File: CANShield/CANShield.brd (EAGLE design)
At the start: 96.5 x 128.3 mm, 69 parts, among them IC1 7805DT, IC2 74LVC2G125DCT, IC3 ILD213T, IC4 ILD213T, IC5 ILD213T, J2 POWERPOLE_POWER25A_HORIZONTAL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, Q1 MOSFET-NCHANNELFDD8780, Q2 MOSFET-NCHANNELFDD8780, Q3 MOSFET-NCHANNELFDD8780, Q4 MOSFET-NCHANNELFDD8780, Q5 MOSFET-NCHANNELFDD8780, Q6 MOSFET-NCHANNELFDD8780, Q7 MOSFET-NCHANNELBSS123LT1G, Q8 BSS123, U5 MCP2551, X1 DB9 Plug

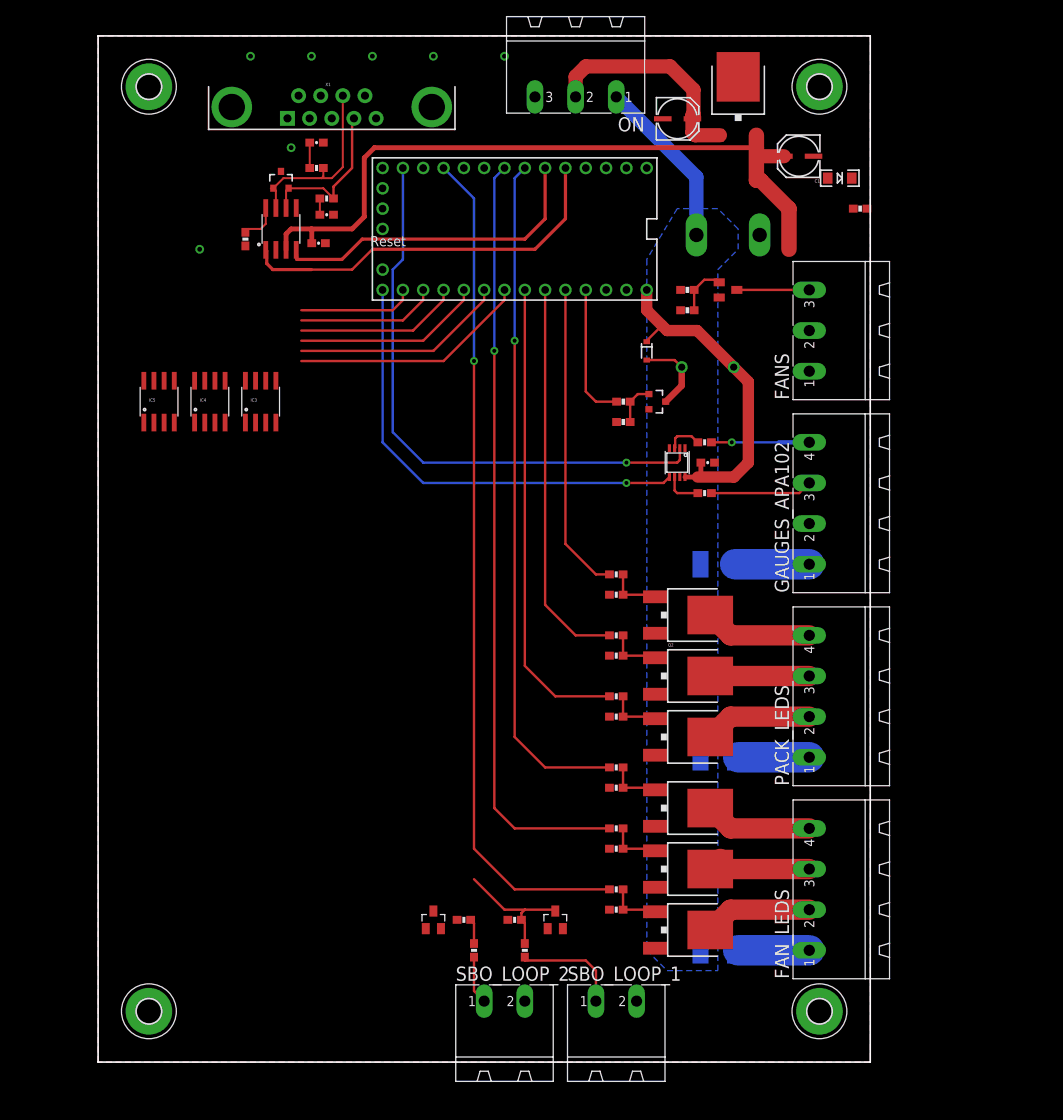
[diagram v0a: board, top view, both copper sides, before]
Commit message: precharge progress
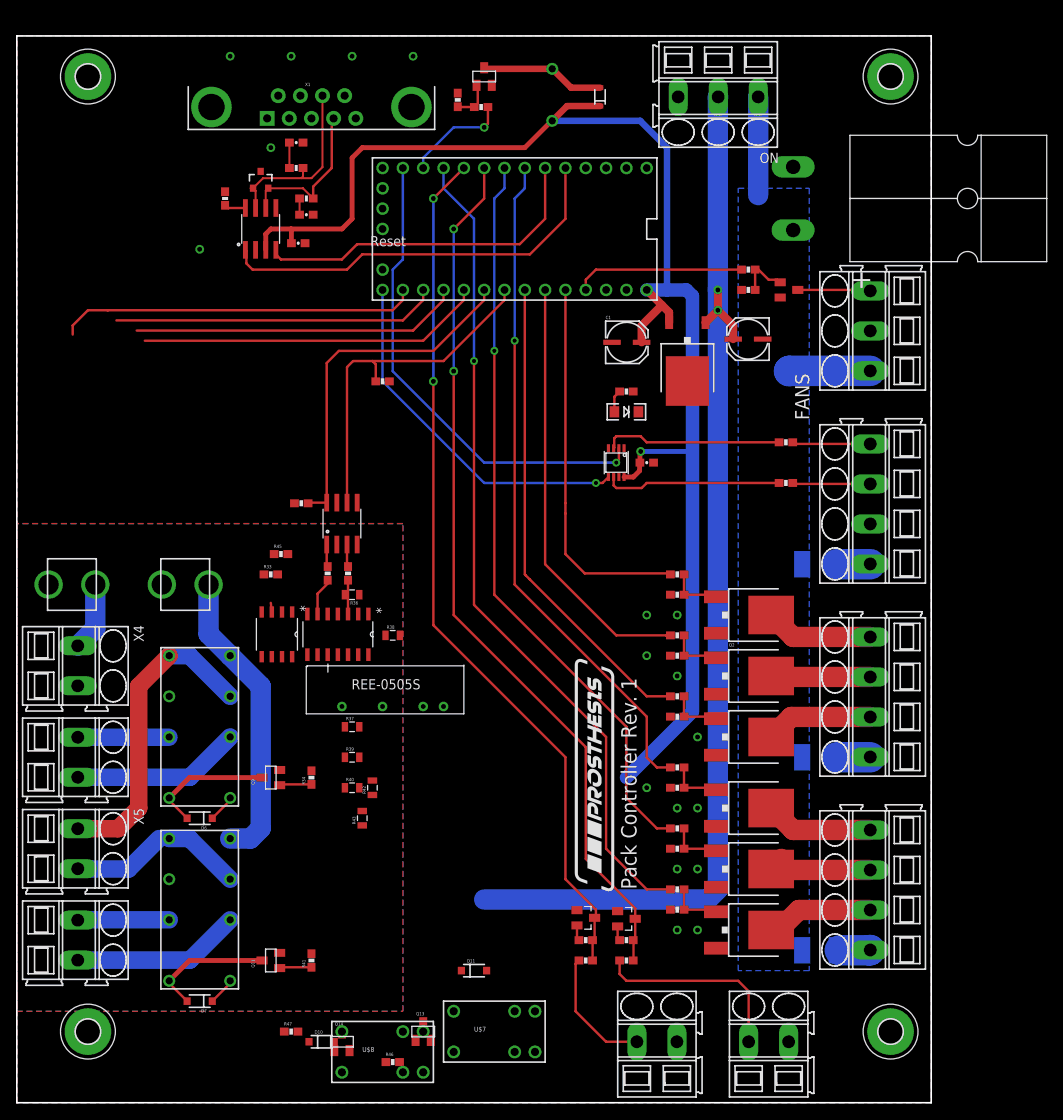
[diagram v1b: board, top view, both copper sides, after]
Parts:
- removed IC4, IC5: ILD213T, SparkFun-DiscreteSemi:SO08
- added 74HC125M: MM74HC125M, Fairchild_By_element14_Batch_1:SOIC127P600X175-14N
- added D10, D11, D6, D7: (no value), SparkFun-DiscreteSemi:SOD-123
- added LM393M: LM393M, Fairchild_By_element14_Batch_1:SOIC127P600X180-8N
- added PRECHARGE_FUSE: FUSEX20MM, SparkFun-Passives:FUSE_5MM
- added PRECHARGE_RELAY, PRECHARGE_RELAY1: DS2Y-S-DC5V, relay:DS2Y
- added Q11, Q13, Q14, Q9: IRLML6344TRPBF, SparkFun-DiscreteSemi:SOT23
- added R23, R24, R25, R26: 10K, SparkFun-Passives:0603-RES
- added R33, R45: 100k, SparkFun-Resistors:0603-RES
- added R34, R41, R46, R47: 10k, SparkFun-Resistors:0603-RES
- added R36, R37, R42: 470k, SparkFun-Resistors:0805
- added R38, R43: 13K, SparkFun-Resistors:0805
- added R39: 110k, SparkFun-Resistors:0805
- added R40: 12K, SparkFun-Resistors:0805
- added U$4: (no value), prosthesis:PROS_LOGO
- added U$5: REE-0505S, grant:REE-0505S
- added U$7, U$8: RELAY-2G5Q, SparkFun-Electromechanical:RELAY-G5V
- added X2, X3, X4, X5: SMKDSP_1,5/2, con-phoenix-smkdsp:SMKDSP_1,5/2
- FANS, ON: value MSTBA3 -> SMKDSP_1,5/3; device con-phoenix-508:MSTBA3 -> con-phoenix-smkdsp:SMKDSP_1,5/3
- FAN_LEDS, GAUGES_APA102, PACK_LEDS: value MSTBA4 -> SMKDSP_1,5/4; device con-phoenix-508:MSTBA4 -> con-phoenix-smkdsp:SMKDSP_1,5/4
- Q7: device SparkFun-DiscreteSemi:SOT23-3 -> SparkFun-DiscreteSemi:SOT23
- R10, R12, R13: device SparkFun-Resistors:0603-RES -> SparkFun-Resistors:0603-RES@1
- SBO_LOOP_1, SBO_LOOP_2: value MSTBA2 -> SMKDSP_1,5/2; device con-phoenix-508:MSTBA2 -> con-phoenix-smkdsp:SMKDSP_1,5/2
- moved Q7 46.0 mm to (44.5, 111.8), turned to 0 degrees
- moved R30 45.3 mm to (41.1, 108.8), turned to 270 degrees
- moved R29 40.9 mm to (44.1, 108.0), turned to 180 degrees
- moved D1 39.6 mm to (62.2, 69.8)
- moved SG1 39.2 mm to (53.0, 109.5), turned to 270 degrees
- moved R22 37.1 mm to (62.2, 72.4), turned to 0 degrees
- moved IC1 33.6 mm to (69.8, 76.2), turned to 180 degrees
- moved D2 32.3 mm to (58.9, 109.2), turned to 90 degrees
- moved C1 31.4 mm to (62.2, 78.7), turned to 0 degrees
- moved C4 29.3 mm to (77.5, 78.7), turned to 180 degrees
- moved ON 20.9 mm to (76.2, 109.2)
- moved D4 19.1 mm to (57.1, 6.60), turned to 270 degrees
- moved SBO_LOOP_1 19.1 mm to (80.0, -8.89)
- moved SBO_LOOP_2 19.1 mm to (66.0, -8.89)
- moved IC3 18.3 mm to (26.7, 55.9)
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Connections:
- removed net CHARGED_1: U$1.18/A4
- removed net CHARGING_1: U$1.19/A5
- new net 96V_IN_FUSED: PRECHARGE_FUSE.1, PRECHARGE_RELAY.8, PRECHARGE_RELAY1.8, R37.2
- new net CAP_CHARGE_REF: LM393M.2, R39.1, R40.2
- new net CAP_CHARGE_V_CURR_1: LM393M.3, R36.1, R38.2
- new net CAP_CHARGE_V_CURR_2: R42.1, R43.2
- new net CHARGE_1: IC3.6, R23.1, U$1.19/A5
- new net CHARGE_2: IC3.8, R26.1, U$1.18/A4
- new net CHARGE_ISO_1: 74HC125M.3, R25.2
- new net CHARGE_ISO_2: 74HC125M.6, R24.2
- new net CONTACT_EN_1: Q13.1, R46.1
- new net CONTACT_EN_2: Q14.1, R47.1
- new net GNDI: IC3.2, IC3.4, U$5.-VOUT, X4.2
- new net N$30: R37.1, R39.2
- new net N$31: 74HC125M.12, 74HC125M.9, LM393M.7, R45.2
- new net N$32: IC3.3, R25.1
- new net N$33: D10.A, Q14.3, U$8.9
- new net N$34: IC3.1, R24.1
- new net N$35: D11.A, Q13.3, U$7.9
- new net N$36: 74HC125M.8
- new net N$37: 74HC125M.11
- new net N$38: U$7.5, U$7.6
- new net N$39: U$8.5, U$8.6
- new net N$40: PRECHARGE_RELAY.13, X2.1
- new net N$41: PRECHARGE_RELAY1.13, X3.1
- new net N$42: PRECHARGE_FUSE.3, X4.1
- new net PRECHARGE_EN_1: Q9.1, R34.1
- new net PRECHARGE_EN_2: Q11.1, R41.1
- new net PRECHARGE_OUT_1: PRECHARGE_RELAY.6, PRECHARGE_RELAY.9, R36.2, X5.1
- new net PRECHARGE_OUT_2: PRECHARGE_RELAY1.6, PRECHARGE_RELAY1.9, R42.2, X5.2
- new net PRECHARGE_RESISTOR_IN: PRECHARGE_RELAY.4, X2.2
- new net PRECHARGE_RESISTOR_IN1: PRECHARGE_RELAY1.4, X3.2
- new net PRECH_DRAIN: D6.A, PRECHARGE_RELAY.16, Q9.3
- new net PRECH_DRAIN1: D7.A, PRECHARGE_RELAY1.16, Q11.3
- new net PRECH_STATE_TO_BUFF: 74HC125M.2, 74HC125M.5, LM393M.1, R33.2
- net +12V: now also D10.C, D11.C, U$7.2, U$8.2
- net +5V: now also R23.2, R26.2, U$5.+VIN
- net 5V: now also 74HC125M.14, D6.C, D7.C, LM393M.8, PRECHARGE_RELAY.1, PRECHARGE_RELAY1.1, R33.1, R45.1, U$5.+VOUT
- net BUZZER: now also U$1.10; no longer U$1.23/A9
- net FAN_PWM: now also U$1.23/A9; no longer U$1.10
- net GND: now also 74HC125M.1, 74HC125M.10, 74HC125M.13, 74HC125M.4, 74HC125M.7, IC3.5, IC3.7, LM393M.4, PRECHARGE_RELAY.11, PRECHARGE_RELAY1.11, Q11.2, Q13.2, Q14.2, Q9.2, R34.2, R38.1, R40.1, R41.2, R43.1, R46.2, R47.2, U$5.-VIN, U$7.10, U$8.10
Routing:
- net VCC: track 28.6 -> 137.9 mm, vias 0 -> 2
- net SBO_SENSE_2: track 3.13 -> 109.4 mm, vias 0 -> 2
- net SBO_SENSE_1: track 16.4 -> 110.2 mm, vias 0 -> 2
- net +5V: track 137.1 -> 182.0 mm, vias 0 -> 1
- net CHARGE_1: track 0.00 -> 44.1 mm
- net CHARGE_2: track 0.00 -> 44.0 mm
- net PRECHARGE_OUT_1: track 0.00 -> 39.0 mm
- net 96V_IN_FUSED: track 0.00 -> 37.5 mm
- net ACTIVE_2: track 14.5 -> 45.0 mm
- net CHARGING_1: track 29.8 -> 0.00 mm
- net CHARGED_1: track 26.8 -> 0.00 mm
- net CHARGED_2: track 17.6 -> 40.7 mm
- net PRECHARGE_OUT_2: track 0.00 -> 22.7 mm
- net PRECHARGE_RESISTOR_IN1: track 0.00 -> 21.1 mm
- net PRECHARGE_RESISTOR_IN: track 0.00 -> 21.1 mm
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- added copper zone on layer 1, net GNDI
- added copper zone on layer 16, net GNDI
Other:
- board size 96.5 x 128.3 mm -> 114.3 x 133.3 mm
- board text added: "Pack Controller Rev. 1"
